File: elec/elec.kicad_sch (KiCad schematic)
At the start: 34 parts, among them J1 Screw terminal, J2 BM04B-SRSS-TB, SW1 YTSA010, U1 MCP23017_SP

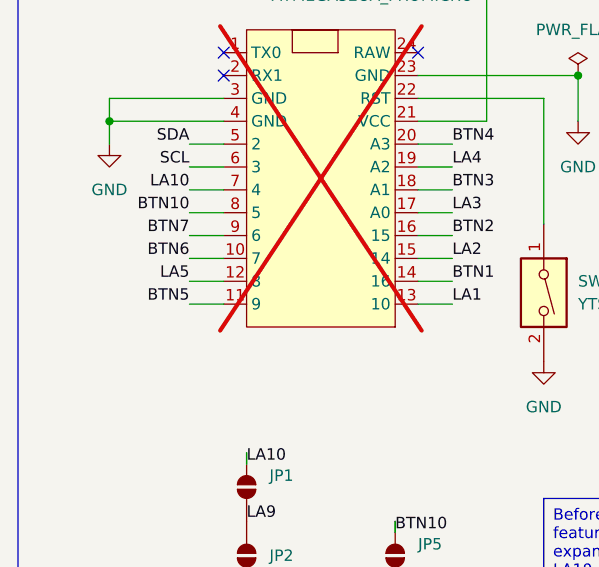
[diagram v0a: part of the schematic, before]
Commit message: main - feat: updating delivrables
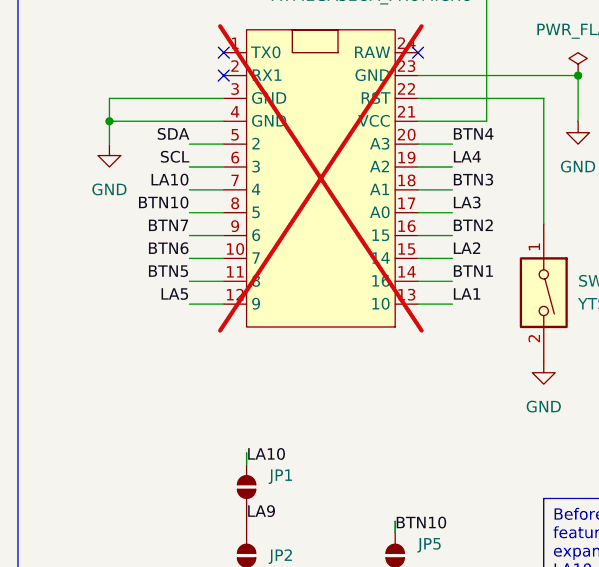
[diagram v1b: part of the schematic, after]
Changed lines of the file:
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@@
 		)
 	)
-	(label "BTN5"
+	(label "LA5"
 		(at 31.75 148.59 180)
 		(fields_autoplaced yes)
@@
 		)
 	)
-	(label "LA5"
+	(label "BTN5"
 		(at 31.75 146.05 180)
 		(fields_autoplaced yes)
